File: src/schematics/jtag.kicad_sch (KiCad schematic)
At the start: 2 parts, among them U6 LFE5U-85F-*BG756*

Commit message: fanout the io connector
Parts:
- R32: footprint Resistor_SMD:R_0603_1608Metric -> Resistor_SMD:R_0402_1005Metric
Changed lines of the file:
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@@
 			)
 		)
-		(property "Footprint" "Resistor_SMD:R_0603_1608Metric"
+		(property "Footprint" "Resistor_SMD:R_0402_1005Metric"
 			(at 146.05 95.25 0)
 			(effects

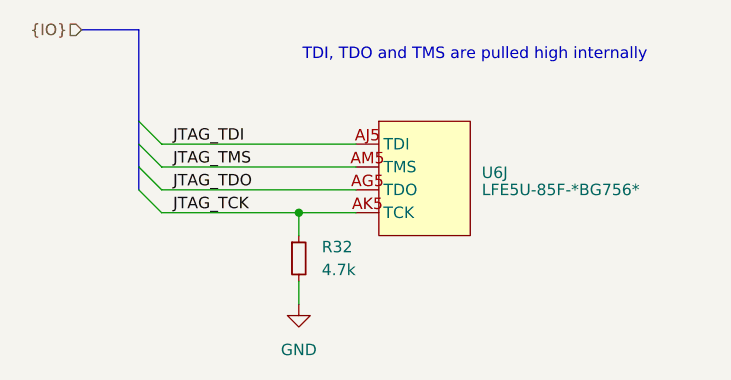
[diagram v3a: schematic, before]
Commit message: Add bom components
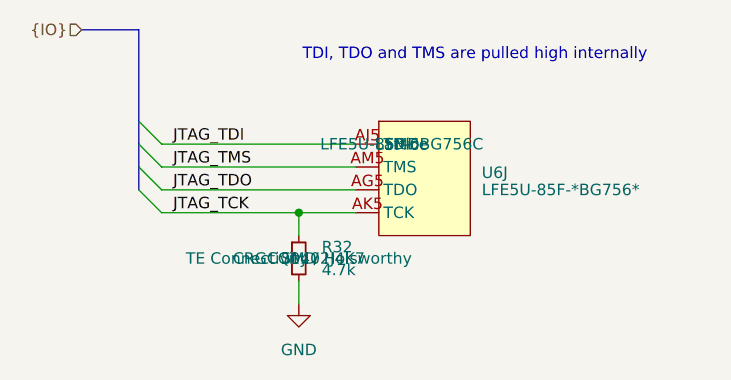
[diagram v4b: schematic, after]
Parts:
- R32: MPN (none) -> CRGCQ0402J4K7; Manufacturer (none) -> TE Connectivity / Holsworthy; Mouting Technology (none) -> SMD
- U6: MPN (none) -> LFE5U-85F-6BG756C; Manufacturer (none) -> Lattice; Mouting Technology (none) -> SMD
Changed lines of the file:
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@@
 			)
 		)
-		(property "Description" "Resistor, small symbol"
-			(at 146.05 95.25 0)
-			(effects
-				(font
-					(size 1.27 1.27)
-				)
-				(hide yes)
+		(property "Description" "4.7k 5% 0402"
+			(at 146.05 95.25 0)
+			(effects
+				(font
+					(size 1.27 1.27)
+				)
+				(hide yes)
+			)
+		)
+		(property "Component" ""
+			(at 146.05 95.25 0)
+			(effects
+				(font
+					(size 1.27 1.27)
+				)
+			)
+		)
+		(property "MPN" "CRGCQ0402J4K7"
+			(at 146.05 95.25 0)
+			(effects
+				(font
+					(size 1.27 1.27)
+				)
+			)
+		)
+		(property "Manufacturer" "TE Connectivity / Holsworthy"
+			(at 146.05 95.25 0)
+			(effects
+				(font
+					(size 1.27 1.27)
+				)
+			)
+		)
+		(property "Sim.Device" ""
+			(at 146.05 95.25 0)
+			(effects
+				(font
+					(size 1.27 1.27)
+				)
+			)
+		)
+		(property "Sim.Type" ""
+			(at 146.05 95.25 0)
+			(effects
+				(font
+					(size 1.27 1.27)
+				)
+			)
+		)
+		(property "Mouting Technology" "SMD"
+			(at 146.05 95.25 0)
+			(effects
+				(font
+					(size 1.27 1.27)
+				)
 			)
 		)
@@
 			)
 		)
+		(property "Component" ""
+			(at 157.48 82.55 0)
+			(effects
+				(font
+					(size 1.27 1.27)
+				)
+			)
+		)
+		(property "MPN" "LFE5U-85F-6BG756C"
+			(at 157.48 82.55 0)
+			(effects
+				(font
+					(size 1.27 1.27)
+				)
+			)
+		)
+		(property "Manufacturer" "Lattice"
+			(at 157.48 82.55 0)
+			(effects
+				(font
+					(size 1.27 1.27)
+				)
+			)
+		)
+		(property "Sim.Device" ""
+			(at 157.48 82.55 0)
+			(effects
+				(font
+					(size 1.27 1.27)
+				)
+			)
+		)
+		(property "Sim.Type" ""
+			(at 157.48 82.55 0)
+			(effects
+				(font
+					(size 1.27 1.27)
+				)
+			)
+		)
+		(property "Mouting Technology" "SMD"
+			(at 157.48 82.55 0)
+			(effects
+				(font
+					(size 1.27 1.27)
+				)
+			)
+		)
